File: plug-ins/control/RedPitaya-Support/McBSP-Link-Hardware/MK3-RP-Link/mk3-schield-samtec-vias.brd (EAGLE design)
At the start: 59.4 x 57.9 mm, 16 parts, among them J4/6 ESQ-122-13-L-T, U1 SN65MLVD202A, U2 SN65MLVD202A, U3 SN65MLVD202A

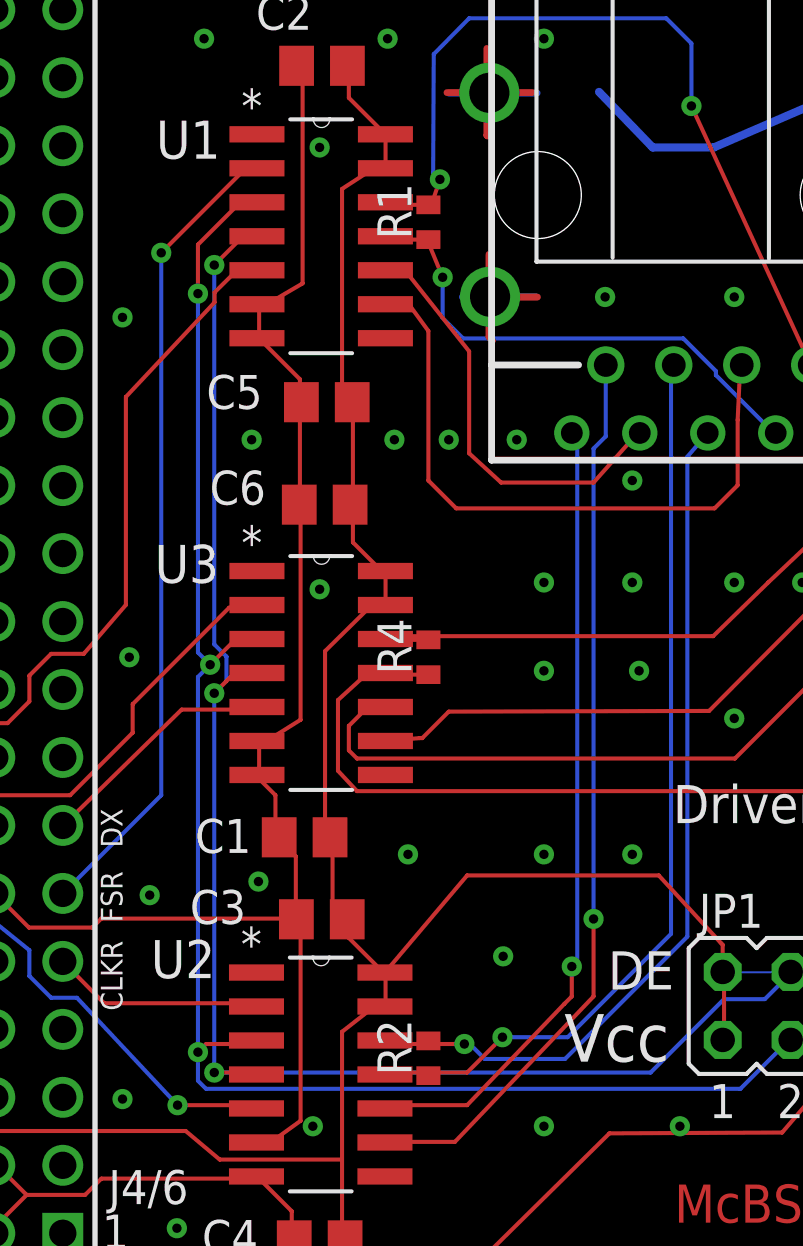
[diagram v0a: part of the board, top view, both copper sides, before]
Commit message: minor updates, cleanups
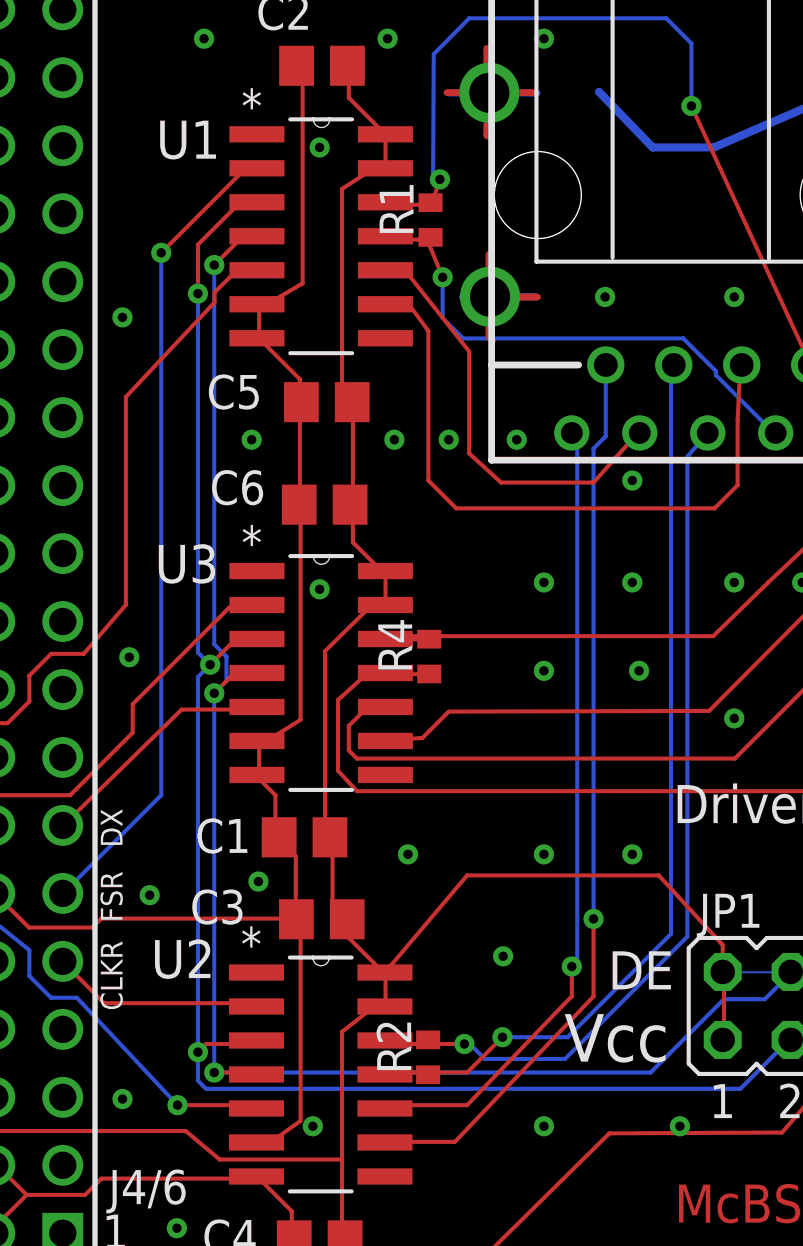
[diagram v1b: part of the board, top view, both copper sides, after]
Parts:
- moved R1 0.11 mm to (23.7, 44.0)
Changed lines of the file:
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@@
 <drawing>
 <settings>
-<setting alwaysvectorfont="no"/>
+<setting alwaysvectorfont="yes"/>
 <setting verticaltext="up"/>
 </settings>
-<grid distance="10" unitdist="mil" unit="mil" style="dots" multiple="1" display="yes" altdistance="0.000123031496" altunitdist="mil" altunit="mil"/>
+<grid distance="0.000123031496" unitdist="mil" unit="mil" style="dots" multiple="1" display="no" altdistance="0.000123031496" altunitdist="mil" altunit="mil"/>
 <layers>
 <layer number="1" name="Top" color="4" fill="1" visible="yes" active="yes"/>
@@
 <attribute name="VALUE" x="12.78513125" y="46.712875" size="1.27" layer="27" rot="R90"/>
 </element>
-<element name="R4" library="resistor" library_urn="urn:adsk.eagle:library:348" package="R0402" package3d_urn="urn:adsk.eagle:package:26058/1" value="100R" x="23.622" y="27.686" rot="R90"/>
-<element name="R1" library="resistor" library_urn="urn:adsk.eagle:library:348" package="R0402" package3d_urn="urn:adsk.eagle:package:26058/1" value="100R" x="23.622" y="43.942" rot="R90"/>
-<element name="R2" library="resistor" library_urn="urn:adsk.eagle:library:348" package="R0402" package3d_urn="urn:adsk.eagle:package:26058/1" value="100R" x="23.622" y="12.7" rot="R90"/>
+<element name="R4" library="resistor" library_urn="urn:adsk.eagle:library:348" package="R0402" package3d_urn="urn:adsk.eagle:package:26058/1" value="100R" x="23.65425625" y="27.71019375" rot="R90"/>
+<element name="R1" library="resistor" library_urn="urn:adsk.eagle:library:348" package="R0402" package3d_urn="urn:adsk.eagle:package:26058/1" value="100R" x="23.703290625" y="44.0233" rot="R90"/>
+<element name="R2" library="resistor" library_urn="urn:adsk.eagle:library:348" package="R0402" package3d_urn="urn:adsk.eagle:package:26058/1" value="100R" x="23.61266875" y="12.73733125" rot="R90"/>
 </elements>
 <signals>
@@
 <wire x1="55.8546" y1="38.6842" x2="55.922" y2="38.607" width="0.1524" layer="1"/>
 <contactref element="R4" pad="2"/>
-<wire x1="23.622" y1="28.336" x2="22.048" y2="28.336" width="0.1524" layer="1"/>
+<wire x1="23.65425625" y1="28.36019375" x2="22.048" y2="28.336" width="0.1524" layer="1"/>
 <wire x1="22.048" y1="28.336" x2="22.017" y2="28.367" width="0.1524" layer="1"/>
 </signal>
@@
 <wire x1="54.6354" y1="35.941" x2="54.652" y2="36.067" width="0.1524" layer="1"/>
 <contactref element="R4" pad="1"/>
-<wire x1="23.622" y1="27.036" x2="22.078" y2="27.036" width="0.1524" layer="1"/>
+<wire x1="23.65425625" y1="27.06019375" x2="22.078" y2="27.036" width="0.1524" layer="1"/>
 <wire x1="22.078" y1="27.036" x2="22.017" y2="27.097" width="0.1524" layer="1"/>
 </signal>
@@
 <wire x1="23.48" y1="44.592" x2="22.112" y2="44.592" width="0.1524" layer="1"/>
 <wire x1="22.112" y1="44.592" x2="22.017" y2="44.687" width="0.1524" layer="1"/>
-<wire x1="23.622" y1="44.592" x2="23.48" y2="44.592" width="0.1524" layer="1"/>
+<wire x1="23.703290625" y1="44.6733" x2="23.48" y2="44.592" width="0.1524" layer="1"/>
 <wire x1="23.48" y1="44.592" x2="23.7998" y2="44.7802" width="0.1524" layer="1"/>
 </signal>
@@
 <via x="24.1554" y="41.8846" extent="1-16" drill="0.35"/>
 <contactref element="R1" pad="1"/>
-<wire x1="23.622" y1="43.292" x2="23.256" y2="43.292" width="0.1524" layer="1"/>
+<wire x1="23.703290625" y1="43.3733" x2="23.256" y2="43.292" width="0.1524" layer="1"/>
 </signal>
 <signal name="N$7">
@@
 <via x="24.9682" y="13.2334" extent="1-16" drill="0.35"/>
 <contactref element="R2" pad="2"/>
-<wire x1="24.9682" y1="13.2334" x2="23.622" y2="13.35" width="0" layer="19" extent="1-16"/>
+<wire x1="24.9682" y1="13.2334" x2="23.61266875" y2="13.38733125" width="0" layer="19" extent="1-16"/>
 </signal>
 <signal name="N$10">
@@
 <via x="26.3906" y="13.4874" extent="1-16" drill="0.35"/>
 <contactref element="R2" pad="1"/>
-<wire x1="25.0698" y1="12.1666" x2="23.622" y2="12.05" width="0" layer="19" extent="1-1"/>
+<wire x1="25.0698" y1="12.1666" x2="23.61266875" y2="12.08733125" width="0" layer="19" extent="1-1"/>
 </signal>
 <signal name="N$11">
